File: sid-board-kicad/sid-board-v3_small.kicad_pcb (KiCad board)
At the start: 2 copper layers, 34.5 x 50.5 mm, 49 parts, among them J1 SPI + UART, J2 USB_B_Micro, J3 UART, Q1 BSS138, Q2 BSS138, SW1 SW_EN, SW2 SW_FLASH, U1 SC16IS752IPW, U2 MCP1703A-3302_SOT223, U3 SN65HVD232, U4 SN65HVD232, U5 CY7C65213-28PVXI, U6 ESP32-WROOM-32U, U7 SN65HVD232, X1 S53305-24.000-X

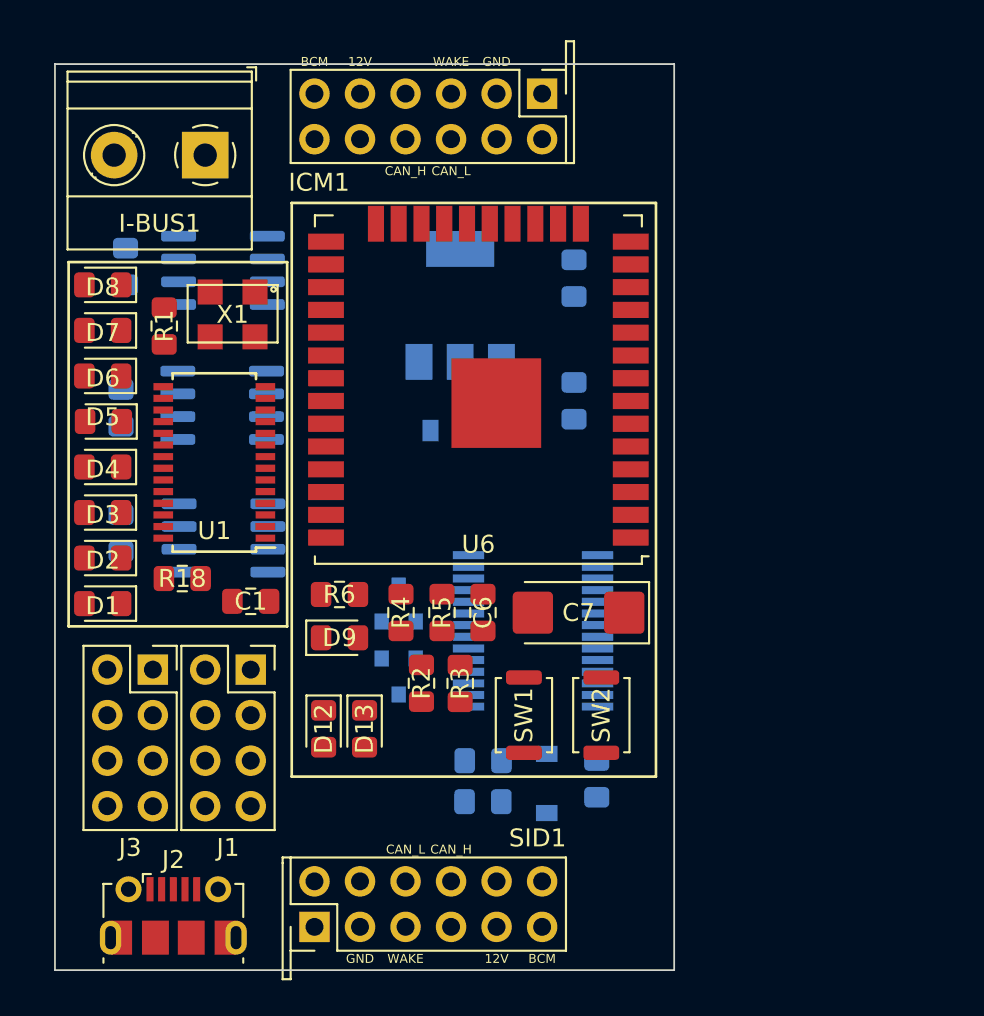
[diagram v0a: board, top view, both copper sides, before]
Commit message: Crazy routing
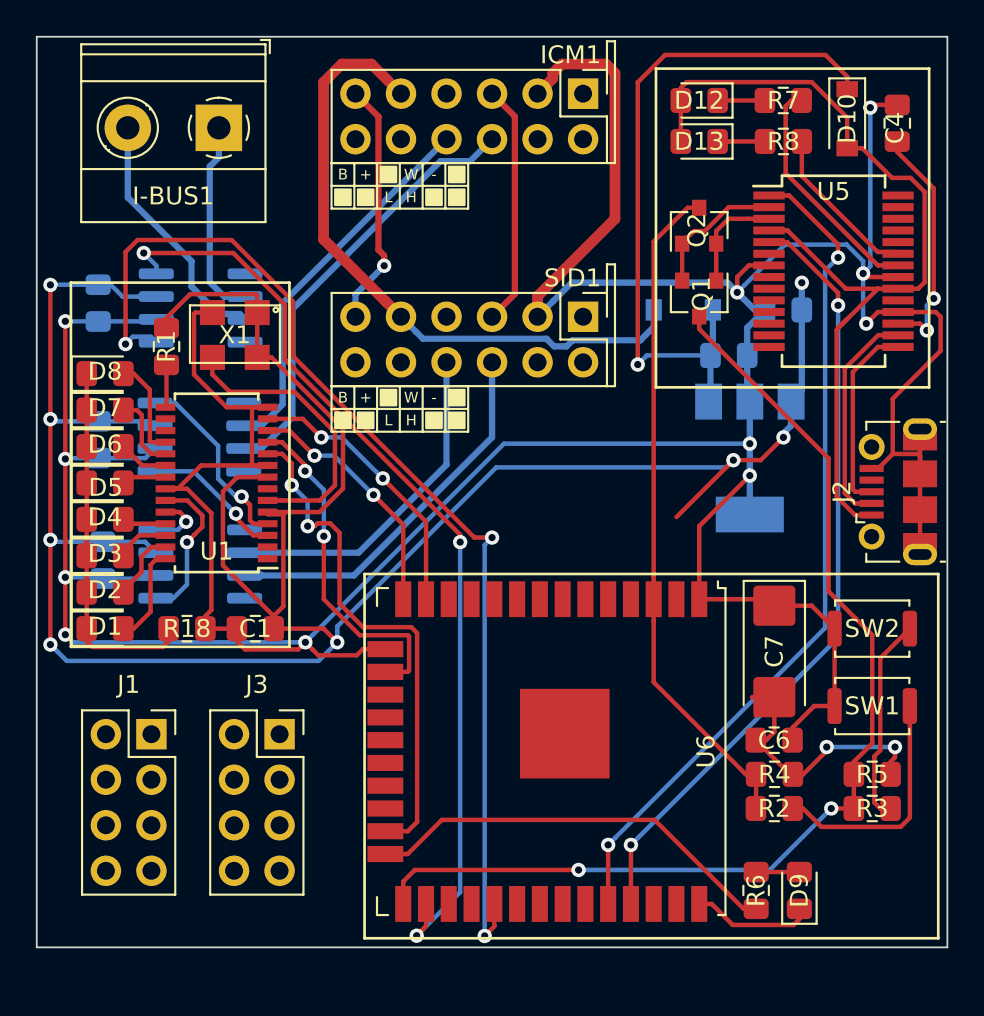
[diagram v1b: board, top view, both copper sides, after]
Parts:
- C4, D10, Q1, Q2, R7, R8, U5: moved to F.Cu
- moved J2 46.8 mm to (116.6, 48.2), turned to 90 degrees
- moved D12 40.8 mm to (105.5, 26.4), turned to 180 degrees
- moved D10 40.7 mm to (113.8, 27.4), turned to 270 degrees
- moved R8 40.5 mm to (110.2, 28.7), turned to 180 degrees
- moved R7 40.5 mm to (110.2, 26.4), turned to 180 degrees
- moved C4 40.2 mm to (116.6, 27.7), turned to 90 degrees
- moved D13 37.7 mm to (105.5, 28.7), turned to 180 degrees
- moved SID1 31.8 mm to (92.7, 39.6), turned to 0 degrees
- moved Q2 30.2 mm to (105.5, 33.4), turned to 90 degrees
- moved D9 29.3 mm to (111.1, 70.5), turned to 90 degrees
- moved R6 28.5 mm to (108.7, 70.5), turned to 270 degrees
- moved U5 26.1 mm to (113.0, 35.9)
- moved R5 25.6 mm to (115.2, 64.0), turned to 180 degrees
- moved R3 24.0 mm to (115.2, 65.9), turned to 0 degrees
- moved Q1 23.9 mm to (105.5, 37.5), turned to 270 degrees
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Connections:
- C2 pad 2: Net-(C2-Pad2) -> GND
- C5 pad 2: Net-(C2-Pad2) -> GND
- ICM1 pad 10: CAN_A_L -> CAN_A_H
- ICM1 pad 9: CAN_A_H -> CAN_A_L
- SID1 pad 10: CAN_B_L -> CAN_B_H
- SID1 pad 9: CAN_B_H -> CAN_B_L
- U2 pad 2: Net-(C2-Pad2) -> GND
- U5 pad 12: SLEEP -> (no net)
- U5 pad 6: RI -> (no net)
- U6 pad 27: RI -> (no net)
- U6 pad 28: SLEEP -> (no net)
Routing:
- net GND: track 0.00 -> 246.6 mm, vias 0 -> 11
- net VDD_3.3V: track 0.00 -> 162.4 mm, vias 0 -> 10
- net TX_ESP32_CAN: track 0.00 -> 60.9 mm, vias 0 -> 3
- net IO0: track 0.00 -> 59.9 mm, vias 0 -> 2
- net RX_ESP32_CAN: track 0.00 -> 52.8 mm, vias 0 -> 3
- net VBUS: track 0.00 -> 51.1 mm
- net RX_ESP32: track 0.00 -> 47.1 mm, vias 0 -> 2
- net TX_ESP32: track 0.00 -> 43.9 mm, vias 0 -> 2
- net VIN: track 0.00 -> 39.6 mm, vias 0 -> 1
- net EN: track 0.00 -> 37.7 mm
- net Net-(D11-Pad2): track 0.00 -> 36.5 mm
- net CS: track 0.00 -> 29.0 mm, vias 0 -> 2
- net CAN_A_H: track 0.00 -> 24.5 mm
- net Net-(R6-Pad2): track 0.00 -> 23.5 mm
- net CAN_A_L: track 0.00 -> 21.2 mm
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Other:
- board size 34.5 x 50.5 mm -> 50.8 x 50.8 mm
